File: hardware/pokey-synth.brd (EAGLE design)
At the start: 120.7 x 69.8 mm, 51 parts, among them IC1 MEGA8-P, IC2 POKEYDIP40, IC3 POKEYDIP40, IC4 6N138

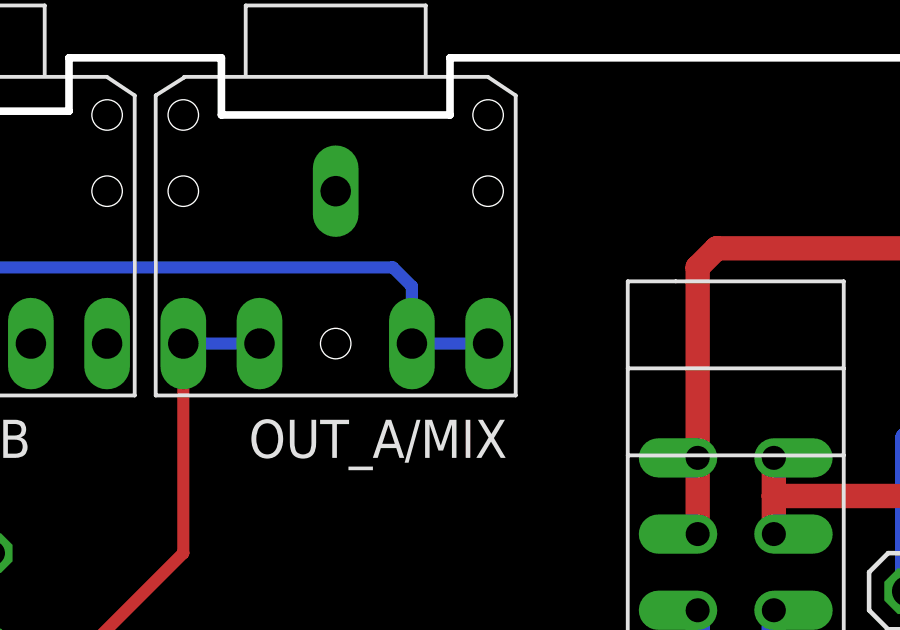
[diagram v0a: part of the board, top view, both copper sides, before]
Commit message: more stuff
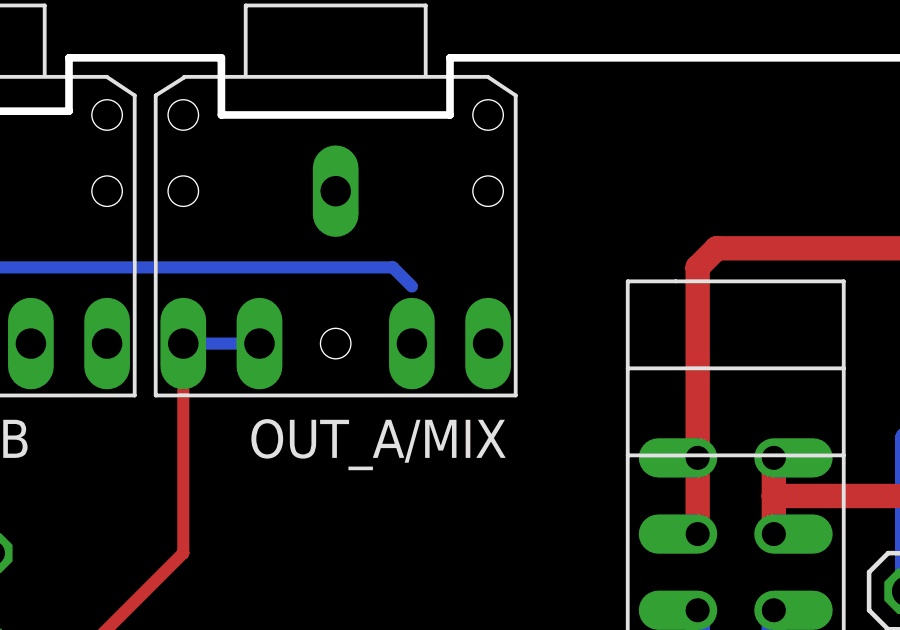
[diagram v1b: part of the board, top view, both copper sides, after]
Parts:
- R6, R7: value (none) -> 470
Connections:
- removed net N$6: OUT_A/MIX.RING, OUT_A/MIX.RING_NC, OUT_B.TIP_NC
- net N$5: now also OUT_B.TIP_NC
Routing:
- net N$6: track 24.7 -> 0.00 mm
- net N$5: track 17.2 -> 37.4 mm
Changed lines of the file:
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@@
 <attribute name="VALUE" x="35.306" y="75.4888" size="1.27" layer="27" ratio="10" rot="R180"/>
 </element>
-<element name="R7" library="rcl" package="0207/7" value="" x="43.815" y="76.2" smashed="yes" rot="R270">
+<element name="R7" library="rcl" package="0207/7" value="470" x="43.815" y="76.2" smashed="yes" rot="R270">
 <attribute name="NAME" x="43.307" y="77.47" size="1.27" layer="25" ratio="10" rot="R270"/>
 <attribute name="VALUE" x="43.2562" y="78.486" size="1.27" layer="27" ratio="10" rot="R270"/>
@@
 <attribute name="NAME" x="14.859" y="62.484" size="1.27" layer="25" ratio="10"/>
 </element>
-<element name="R6" library="rcl" package="0207/7" value="" x="40.64" y="76.2" smashed="yes" rot="R270">
+<element name="R6" library="rcl" package="0207/7" value="470" x="40.64" y="76.2" smashed="yes" rot="R270">
 <attribute name="NAME" x="40.132" y="77.47" size="1.27" layer="25" ratio="10" rot="R270"/>
 <attribute name="VALUE" x="40.0812" y="78.486" size="1.27" layer="27" ratio="10" rot="R270"/>
@@
 <wire x1="87.63" y1="82.55" x2="84.455" y2="79.375" width="0.4064" layer="1"/>
 <wire x1="81.28" y1="79.375" x2="84.455" y2="79.375" width="0.4064" layer="1"/>
-</signal>
-<signal name="N$6">
-<contactref element="OUT_A/MIX" pad="RING"/>
-<contactref element="OUT_A/MIX" pad="RING_NC"/>
 <contactref element="OUT_B" pad="TIP_NC"/>
-<wire x1="95.25" y1="89.535" x2="97.79" y2="89.535" width="0.4064" layer="16"/>
 <wire x1="94.615" y1="92.075" x2="78.105" y2="92.075" width="0.4064" layer="16"/>
 <wire x1="78.105" y1="92.075" x2="77.47" y2="91.44" width="0.4064" layer="16"/>
 <wire x1="77.47" y1="91.44" x2="77.47" y2="89.535" width="0.4064" layer="16"/>
-<wire x1="95.25" y1="89.535" x2="95.25" y2="91.44" width="0.4064" layer="16"/>
 <wire x1="95.25" y1="91.44" x2="94.615" y2="92.075" width="0.4064" layer="16"/>
+<wire x1="90.17" y1="89.535" x2="94.615" y2="92.075" width="0" layer="19" extent="16-16"/>
 </signal>
 <signal name="N$7">
